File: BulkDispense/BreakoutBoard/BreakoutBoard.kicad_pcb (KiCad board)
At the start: 2 copper layers, 70 x 102.5 mm, 26 parts, among them J1 Power Source, J10 BS2, J11 BS4, J12 OS1, J13 OS3, J14 Analog Inputs, J15 Digital IN + R0~R4, J16 Digital Outputs, J17 R4~R9, J18 OS2, J19 OS4, J2 WL1, J20 PS, J21 PCV, J22 MV1&2, J23 R0~R3, J24 MV3&4, J25 R4~R7, J26 R8~R9, J3 WB1, J4 WV1, J5 WL2, J6 BS1, J7 BS3, J8 WB2, J9 WV2

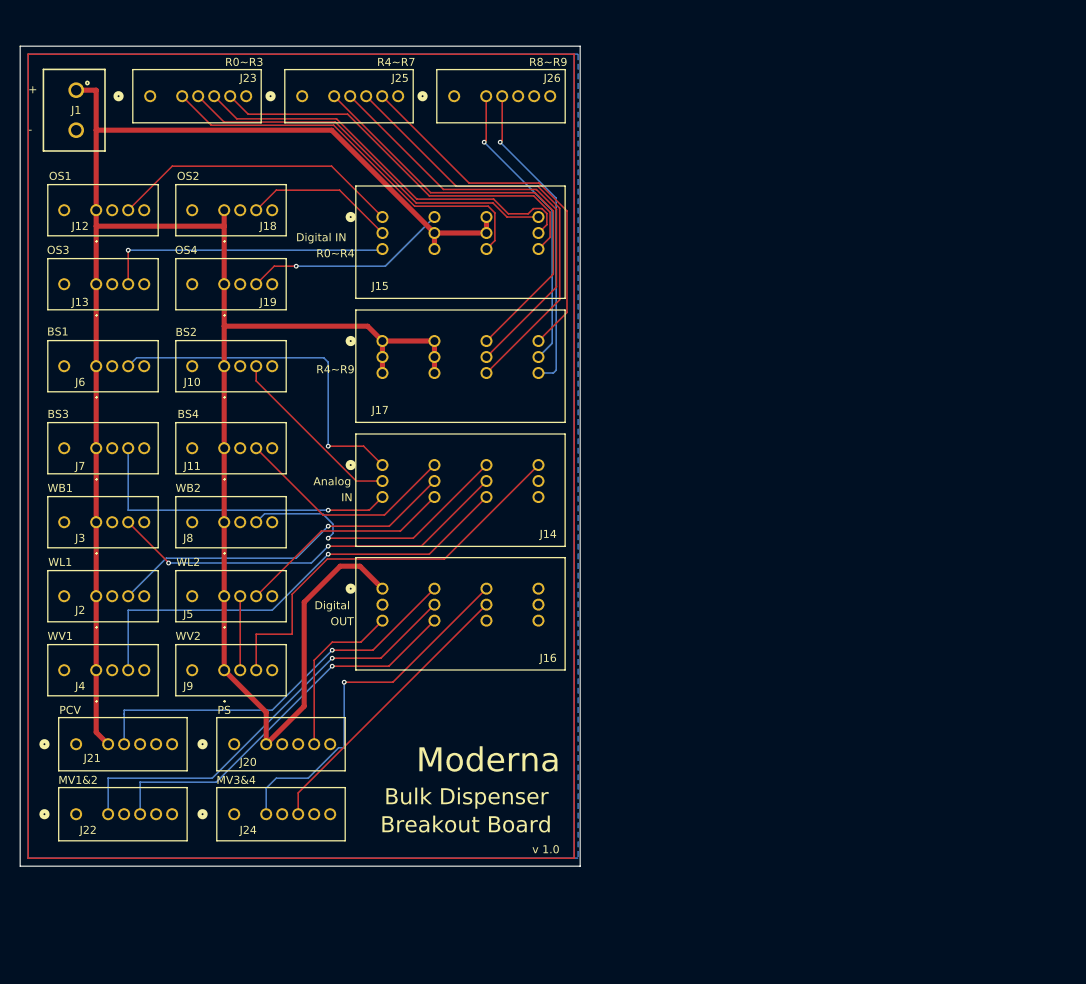
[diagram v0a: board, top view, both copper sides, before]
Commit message: Add more documentation + holding mounts
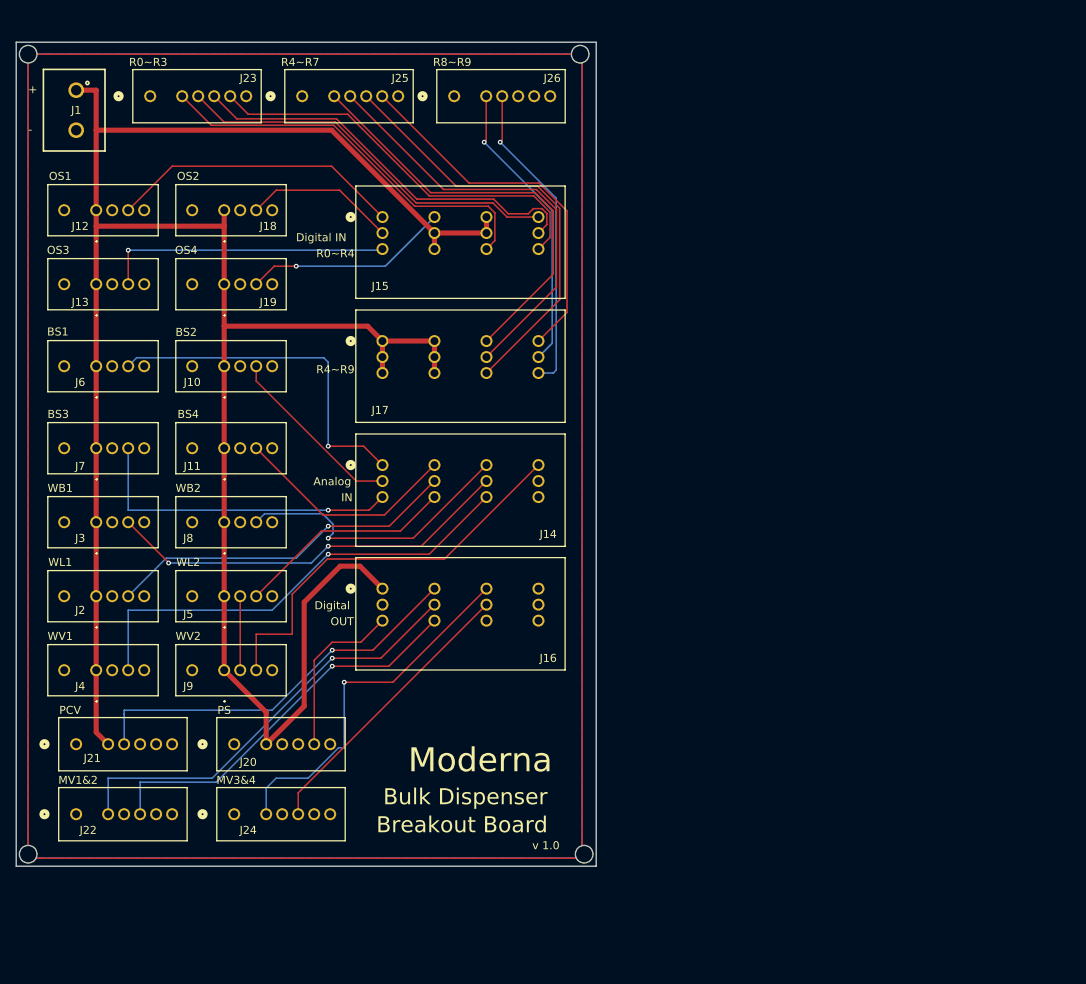
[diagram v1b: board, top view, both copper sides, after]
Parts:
- added H1: MountingHole, MountingHole:MountingHole_2.2mm_M2, F.Cu at (120.5, 37.0)
- added H2: MountingHole, MountingHole:MountingHole_2.2mm_M2, F.Cu at (51.5, 37.0)
- added H3: MountingHole, MountingHole:MountingHole_2.2mm_M2, F.Cu at (121.0, 137.0)
- added H4: MountingHole, MountingHole:MountingHole_2.2mm_M2, F.Cu at (51.5, 137.0)
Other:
- board size 70 x 102.5 mm -> 72.5 x 103 mm

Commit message: Finished Up Board + MAXIExpansionBoard
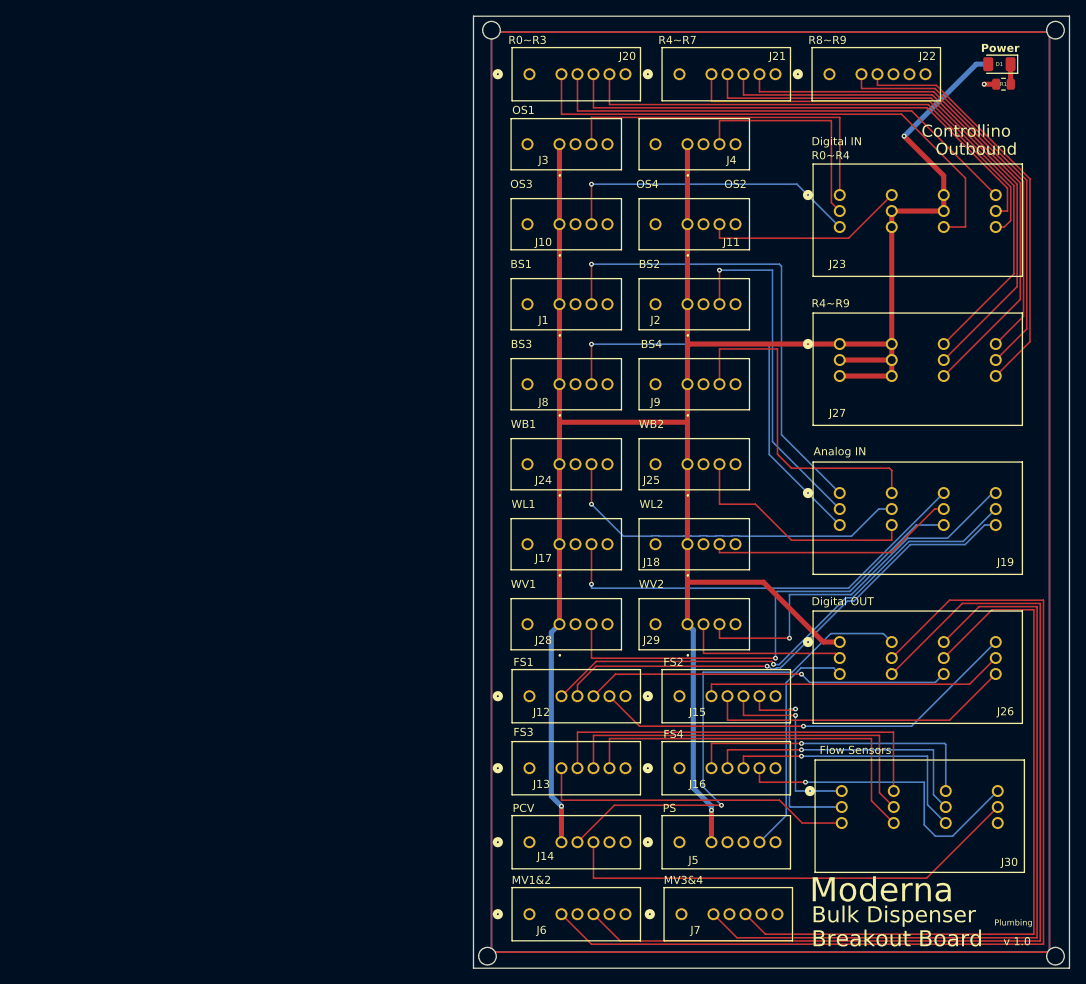
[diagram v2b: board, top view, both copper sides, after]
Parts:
- removed the J1 at (57.5, 44.0)
- added D1: LED, LED_SMD:LED_1206_3216Metric, F.Cu at (172.9, 38.2)
- added J12: FS1, PartsLibrary:CONN_37204-62A3-004PL_3MM, F.Cu at (118.2, 117.2)
- added J13: FS3, PartsLibrary:CONN_37204-62A3-004PL_3MM, F.Cu at (118.2, 126.2)
- added J15: FS2, PartsLibrary:CONN_37204-62A3-004PL_3MM, F.Cu at (136.9, 117.2)
- added J16: FS4, PartsLibrary:CONN_37204-62A3-004PL_3MM, F.Cu at (136.9, 126.2)
- added J30: Flow Sensors, PartsLibrary:CONN_37212-62M3-003PL_3MM, F.Cu at (153.2, 129.1)
- added R1: R, Resistor_SMD:R_0805_2012Metric, F.Cu at (173.4, 40.8)
- moved H4 129.0 mm to (179.9, 149.8)
- moved H2 128.4 mm to (179.9, 34.0)
- moved J3 58.5 mm to (117.9, 48.2)
- moved J4 58.5 mm to (133.9, 48.2)
- moved J8 58.5 mm to (117.9, 78.2)
- moved J9 58.5 mm to (133.9, 78.2)
- moved J1 58.4 mm to (117.9, 68.2)
- moved J2 58.4 mm to (133.9, 68.2)
- moved J10 58.4 mm to (117.9, 58.2)
- moved J11 58.4 mm to (133.9, 58.2)
- moved J24 58.4 mm to (117.9, 88.2)
- moved J25 58.4 mm to (133.9, 88.2)
- moved J17 58.3 mm to (117.9, 98.2)
- moved J18 58.3 mm to (133.9, 98.2)
- moved J28 58.2 mm to (117.9, 108.2)
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- renumbered J6 to J1, J13 to J10, J19 to J11, J21 to J14, J2 to J17, J5 to J18, J14 to J19, J10 to J2, J23 to J20, J25 to J21, J26 to J22, J15 to J23, J3 to J24, J8 to J25, J16 to J26, J17 to J27, J4 to J28, J9 to J29, J12 to J3, J18 to J4, J20 to J5, J22 to J6, J24 to J7, J7 to J8, J11 to J9
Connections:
- J17 pad 3: /AI4 -> /AI6
- J18 pad 3: /AI5 -> /AI7
- J19 pad 11: /AI10 -> /FS1-1
- J19 pad 12: /AI11 -> /FS1-2
- J24 pad 3: /AI7 -> /AI4
- J25 pad 3: /AI6 -> /AI5
- J26 pad 10: /DO5 -> /FS1-4
- J26 pad 11: /DO6 -> /FS2-1
- J26 pad 12: /DO7 -> /FS2-2
- J26 pad 9: /DO4 -> /FS1-3
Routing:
- net /DO1: track 49.2 -> 121.7 mm, vias 1 -> 0
- net /DO0: track 54.3 -> 126.8 mm, vias 1 -> 0
- net /FS1-1: track 0.00 -> 64.4 mm, vias 0 -> 1
- net /FS1-2: track 0.00 -> 62.3 mm, vias 0 -> 1
- net /AO0: track 0.00 -> 58.7 mm
- net /DO3: track 35.9 -> 91.4 mm
- net /FS1-4: track 0.00 -> 54.2 mm, vias 0 -> 1
- net /FS3-2: track 0.00 -> 51.4 mm
- net /DO2: track 45.9 -> 96.6 mm, vias 1 -> 0
- net /FS3-3: track 0.00 -> 49.5 mm
- net /FS3-4: track 0.00 -> 48.2 mm
- net /FS1-3: track 0.00 -> 45.8 mm, vias 0 -> 1
- net /FS3-1: track 0.00 -> 40.2 mm
- net /FS4-4: track 0.00 -> 39.8 mm, vias 0 -> 1
- net /FS2-2: track 0.00 -> 38.9 mm
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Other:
- board size 72.5 x 103 mm -> 74.5 x 119 mm
- board text added: "Analog IN"
- board text added: "Controllino"
- board text added: "Digital OUT"
- board text added: "Outbound"
- board text added: "Plumbing"
- board text added: "Power"
- board text removed: "+"
- board text removed: "-"
- board text removed: "Analog"
- board text removed: "Digital"
- board text removed: "IN"
- board text removed: "OUT"
